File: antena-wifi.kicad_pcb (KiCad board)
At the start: 2 copper layers, 40.6 x 52.3 mm, 19 parts, among them J1 Conn_01x01, J2 USB_C_Receptacle_USB2.0, SW1 Sw_Res

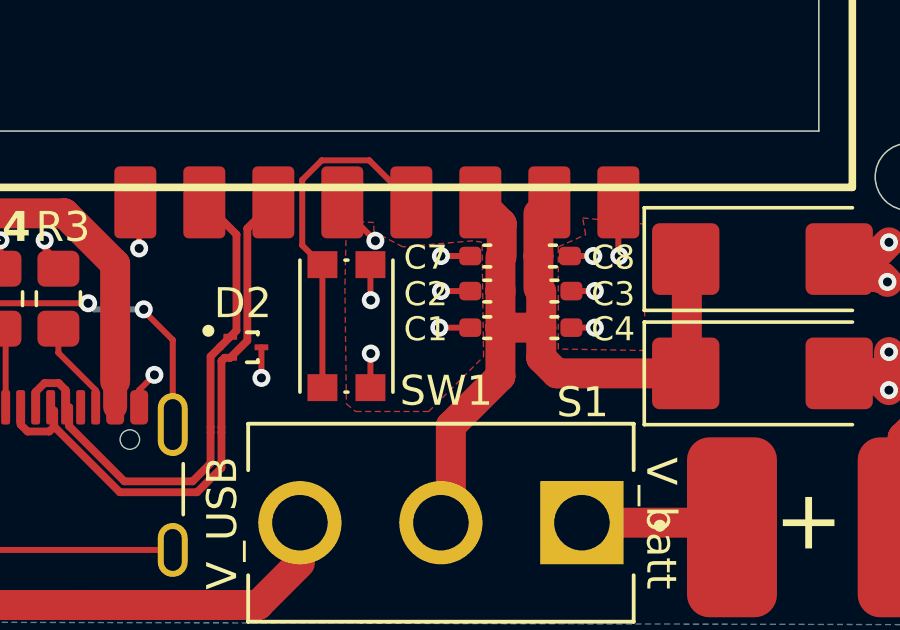
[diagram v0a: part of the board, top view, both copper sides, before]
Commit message: mała poprawka z gnd
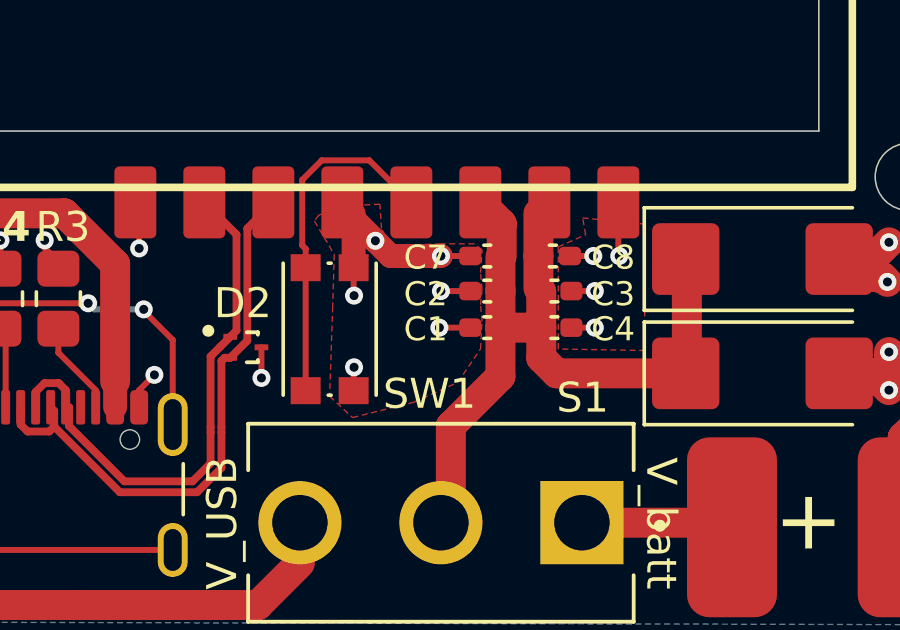
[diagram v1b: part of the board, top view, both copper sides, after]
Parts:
- moved SW1 0.57 mm to (102.6, 147.3)
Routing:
- net GND: track 47.9 -> 52.0 mm
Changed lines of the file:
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@@
 	(footprint "Button_Switch_SMD:SW_Push_1P1T_NO_CK_KMR2"
 		(layer "F.Cu")
-		(at 103.1748 147.2184 -90)
+		(at 102.616 147.32 -90)
 		(descr "CK components KMR2 tactile switch http://www.ckswitches.com/media/1479/kmr2.pdf")
 		(tags "tactile switch kmr2")
@@
 		(at 106.3244 153.7716 180)
 		(property "Reference" "S1"
-			(at -4.7244 4.0132 180)
+			(at -4.7244 4.1656 180)
 			(layer "F.SilkS")
 			(effects
@@
 	)
 	(gr_text "SW1"
-		(at 104.9528 149.9616 0)
+		(at 104.394 150.0632 0)
 		(layer "F.SilkS")
 		(effects
@@
 	)
 	(segment
+		(start 103.416 145.27)
+		(end 103.416 146.1896)
+		(width 0.2)
+		(layer "F.Cu")
+		(net 2)
+	)
+	(segment
 		(start 96.774 148.844)
 		(end 96.2656 149.3524)
@@
 	)
 	(segment
+		(start 103.416 149.37)
+		(end 103.416 148.6028)
+		(width 0.2)
+		(layer "F.Cu")
+		(net 2)
+	)
+	(segment
 		(start 103.0384 143.0936)
 		(end 103.0384 143.272)
@@
 	)
 	(segment
-		(start 103.9748 145.1684)
-		(end 103.9748 146.342)
-		(width 0.2)
-		(layer "F.Cu")
-		(net 2)
-	)
-	(segment
 		(start 93.1164 144.3592)
 		(end 93.1164 144.6132)
@@
 	)
 	(segment
+		(start 103.416 146.1896)
+		(end 103.4288 146.2024)
+		(width 0.2)
+		(layer "F.Cu")
+		(net 2)
+	)
+	(segment
 		(start 110.6739 146.05)
 		(end 111.4552 146.05)
@@
 	)
 	(segment
-		(start 103.9748 149.2684)
-		(end 103.9748 148.1456)
+		(start 96.266 144.6276)
+		(end 96.266 143.2212)
 		(width 0.2)
 		(layer "F.Cu")
@@
 	)
 	(segment
-		(start 96.266 144.6276)
-		(end 96.266 143.2212)
-		(width 0.2)
+		(start 106.3244 144.8816)
+		(end 104.648 144.8816)
+		(width 0.8)
 		(layer "F.Cu")
 		(net 2)
@@
 	)
 	(segment
-		(start 112.2384 143.0936)
-		(end 112.2384 144.852)
-		(width 0.2)
+		(start 103.416 145.27)
+		(end 103.416 143.4712)
+		(width 0.8)
 		(layer "F.Cu")
 		(net 2)
 	)
 	(segment
-		(start 96.2656 149.3524)
-		(end 96.2656 149.9244)
+		(start 112.2384 143.0936)
+		(end 112.2384 144.852)
 		(width 0.2)
 		(layer "F.Cu")
@@
 	)
 	(segment
-		(start 103.9748 146.342)
-		(end 103.9876 146.3548)
+		(start 96.2656 149.3524)
+		(end 96.2656 149.9244)
 		(width 0.2)
 		(layer "F.Cu")
@@
 	)
 	(segment
-		(start 103.0384 143.272)
-		(end 104.14 144.3736)
+		(start 103.416 143.4712)
+		(end 103.0384 143.0936)
 		(width 0.2)
 		(layer "F.Cu")
@@
 	)
 	(segment
-		(start 103.9748 148.1456)
-		(end 103.9876 148.1328)
-		(width 0.2)
+		(start 103.0384 143.272)
+		(end 104.14 144.3736)
+		(width 0.8)
 		(layer "F.Cu")
 		(net 2)
@@
 	)
 	(segment
+		(start 104.648 144.8816)
+		(end 104.14 144.3736)
+		(width 0.8)
+		(layer "F.Cu")
+		(net 2)
+	)
+	(segment
 		(start 121.7168 151.4348)
 		(end 121.7168 153.924)
@@
 		(net 2)
 	)
+	(segment
+		(start 103.416 148.6028)
+		(end 103.4288 148.59)
+		(width 0.2)
+		(layer "F.Cu")
+		(net 2)
+	)
 	(via
 		(at 88.5952 145.6436)
@@
 	)
 	(via
-		(at 96.266 144.6276)
+		(at 103.4288 146.2024)
 		(size 0.6)
 		(drill 0.3)
@@
 	)
 	(via
-		(at 122.2248 150.4188)
+		(at 96.266 144.6276)
 		(size 0.6)
 		(drill 0.3)
@@
 	)
 	(via
-		(at 91.6432 144.3592)
+		(at 122.2248 150.4188)
 		(size 0.6)
 		(drill 0.3)
@@
 	)
 	(via
-		(at 103.9876 146.3548)
+		(at 91.6432 144.3592)
 		(size 0.6)
 		(drill 0.3)
 		(layers "F.Cu" "B.Cu")
-		(free yes)
 		(net 2)
 	)
@@
 	)
 	(via
-		(at 103.9876 148.1328)
+		(at 87.5384 130.7692)
 		(size 0.6)
 		(drill 0.3)
 		(layers "F.Cu" "B.Cu")
-		(free yes)
 		(net 2)
 	)
 	(via
-		(at 87.5384 130.7692)
+		(at 106.3244 144.8816)
 		(size 0.6)
 		(drill 0.3)
 		(layers "F.Cu" "B.Cu")
+		(free yes)
 		(net 2)
 	)
 	(via
-		(at 106.3244 144.8816)
+		(at 103.4288 148.59)
 		(size 0.6)
 		(drill 0.3)
 		(layers "F.Cu" "B.Cu")
-		(free yes)
 		(net 2)
 	)
@@
 	)
 	(segment
-		(start 102.3748 145.1684)
-		(end 102.344 145.1684)
+		(start 103.9374 141.6926)
+		(end 105.3384 143.0936)
 		(width 0.2)
 		(layer "F.Cu")
@@
 	)
 	(segment
-		(start 103.9374 141.6926)
-		(end 105.3384 143.0936)
+		(start 101.816 149.37)
+		(end 101.816 145.27)
 		(width 0.2)
 		(layer "F.Cu")
@@
 	)
 	(segment
-		(start 101.7016 142.343806)
-		(end 102.352806 141.6926)
+		(start 101.816 145.27)
+		(end 101.816 144.6404)
 		(width 0.2)
 		(layer "F.Cu")
@@
 	)
 	(segment
-		(start 102.3748 149.2684)
-		(end 102.3748 145.1684)
+		(start 101.816 144.6404)
+		(end 101.7016 144.526)
 		(width 0.2)
 		(layer "F.Cu")
@@
 	)
 	(segment
-		(start 102.344 145.1684)
-		(end 101.7016 144.526)
+		(start 101.7016 142.343806)
+		(end 102.352806 141.6926)
 		(width 0.2)
 		(layer "F.Cu")
@@
 		(polygon
 			(pts
-				(xy 103.1748 143.7132) (xy 103.124 145.9484) (xy 103.1748 149.8092) (xy 103.4796 150.0632) (xy 105.918 150.0632)
-				(xy 107.7468 148.2344) (xy 107.696 144.4244) (xy 107.3912 144.3736) (xy 105.0544 144.5768) (xy 104.0892 144.0688)
-				(xy 104.0892 143.764)
+				(xy 102.108 143.7132) (xy 102.7684 144.8308) (xy 102.7176 146.558) (xy 102.616 149.5552) (xy 103.378 150.2664)
+				(xy 105.41 149.7584) (xy 106.8832 149.098) (xy 107.6452 147.9804) (xy 107.696 147.066) (xy 107.6452 146.5072)
+				(xy 107.696 145.9992) (xy 107.6452 145.4404) (xy 107.696 144.6784) (xy 107.442 144.4752) (xy 106.3244 144.4752)
+				(xy 104.9528 144.526) (xy 104.5972 144.4752) (xy 104.3432 143.9672) (xy 104.2924 143.1544) (xy 103.2764 143.2052)
+				(xy 102.2604 143.51)
 			)
 		)
